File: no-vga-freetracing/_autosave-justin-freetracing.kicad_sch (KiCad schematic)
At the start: 121 parts, among them J1 DB15_Female_HighDensity, J2 Conn_02x03_Odd_Even, J3 Conn_01x08_MountingPin, J5 Barrel_Jack_Switch_Pin3Ring, K1 SW_Push, K10 SW_Push, K11 SW_Push, K12 SW_Push, K13 SW_Push, K14 SW_Push, K15 SW_Push, K16 SW_Push, K17 SW_Push, K18 SW_Push, K19 SW_Push, K2 SW_Push, K20 SW_Push, K21 SW_Push, K22 SW_Push, K23 SW_Push, K24 SW_Push, K25 SW_Push, K26 SW_Push, K27 SW_Push, K28 SW_Push, K29 SW_Push, K3 SW_Push, K30 SW_Push, K31 SW_Push, K32 SW_Push, K33 SW_Push, K34 SW_Push, K35 SW_Push, K36 SW_Push, K37 SW_Push, K38 SW_Push, K39 SW_Push, K4 SW_Push, K40 SW_Push, K41 SW_Push, K42 SW_Push, K43 SW_Push, K44 SW_Push, K45 SW_Push, K46 SW_Push, K47 SW_Push, K48 SW_Push, K49 SW_Push, K5 SW_Push, K6 SW_Push, K7 SW_Push, K8 SW_Push, K9 SW_Push, U1 ATmega1284-P, U2 ICE40UL1K-SWG16, Y1 20MHz

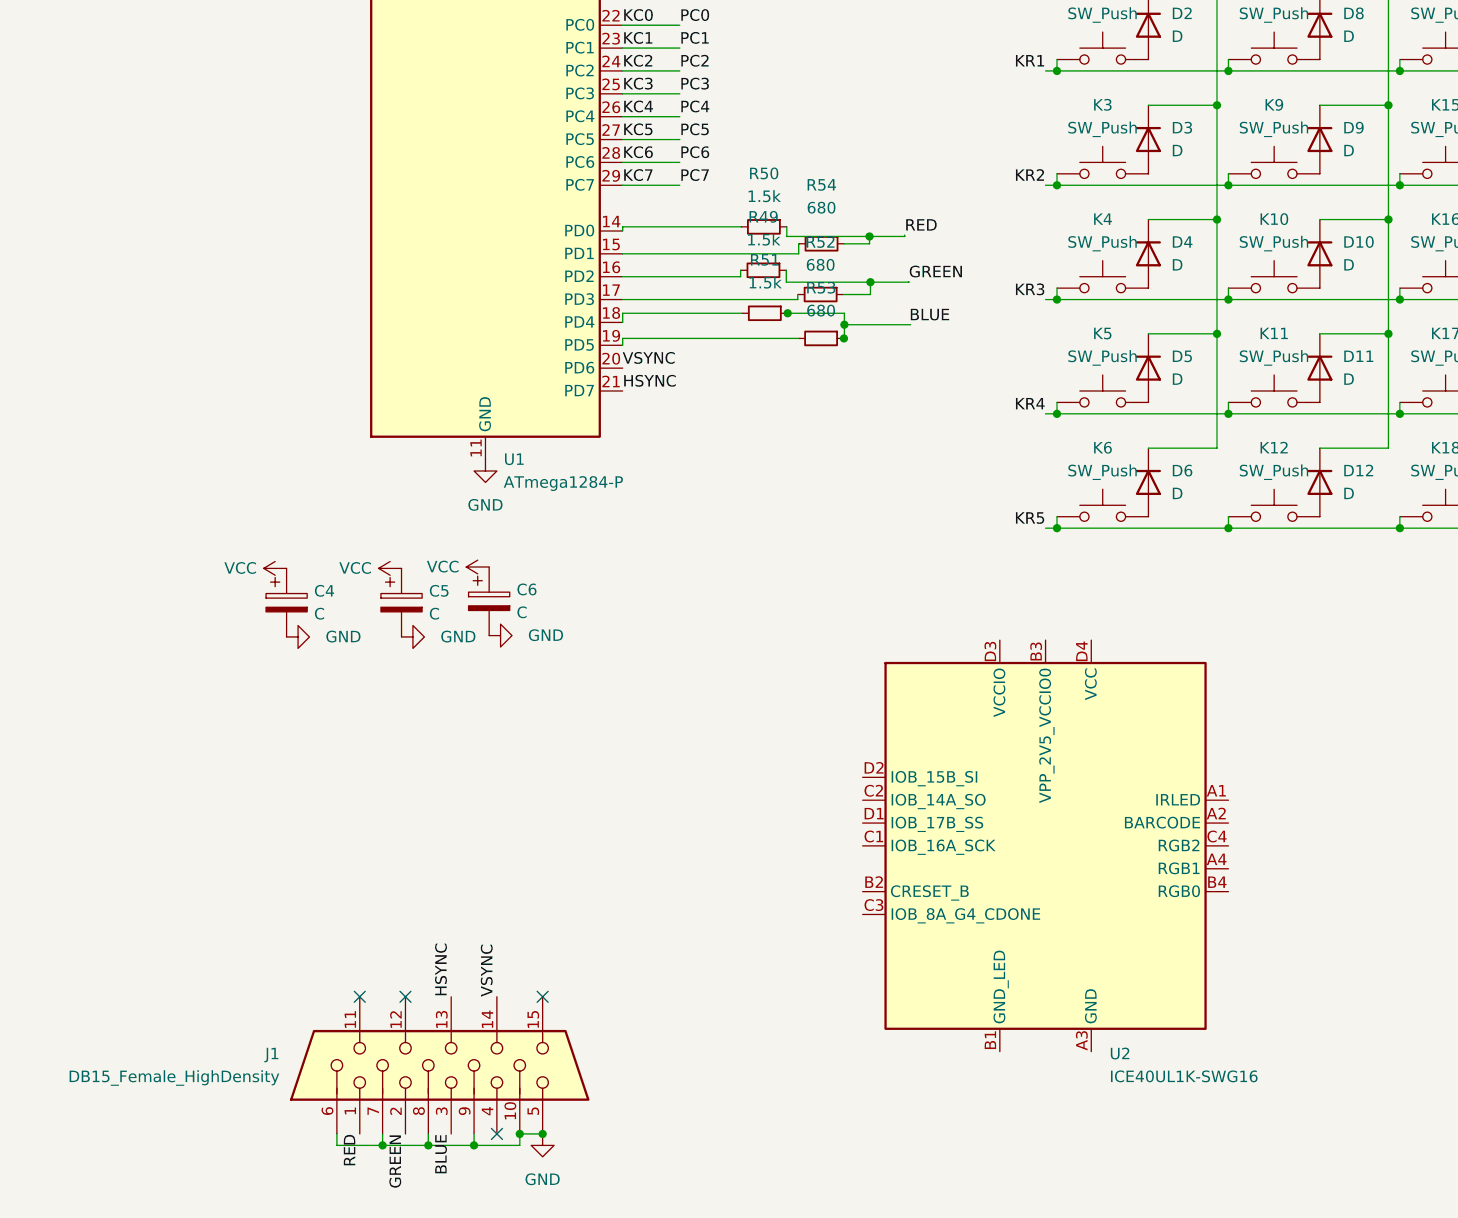
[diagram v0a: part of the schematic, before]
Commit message: Additional
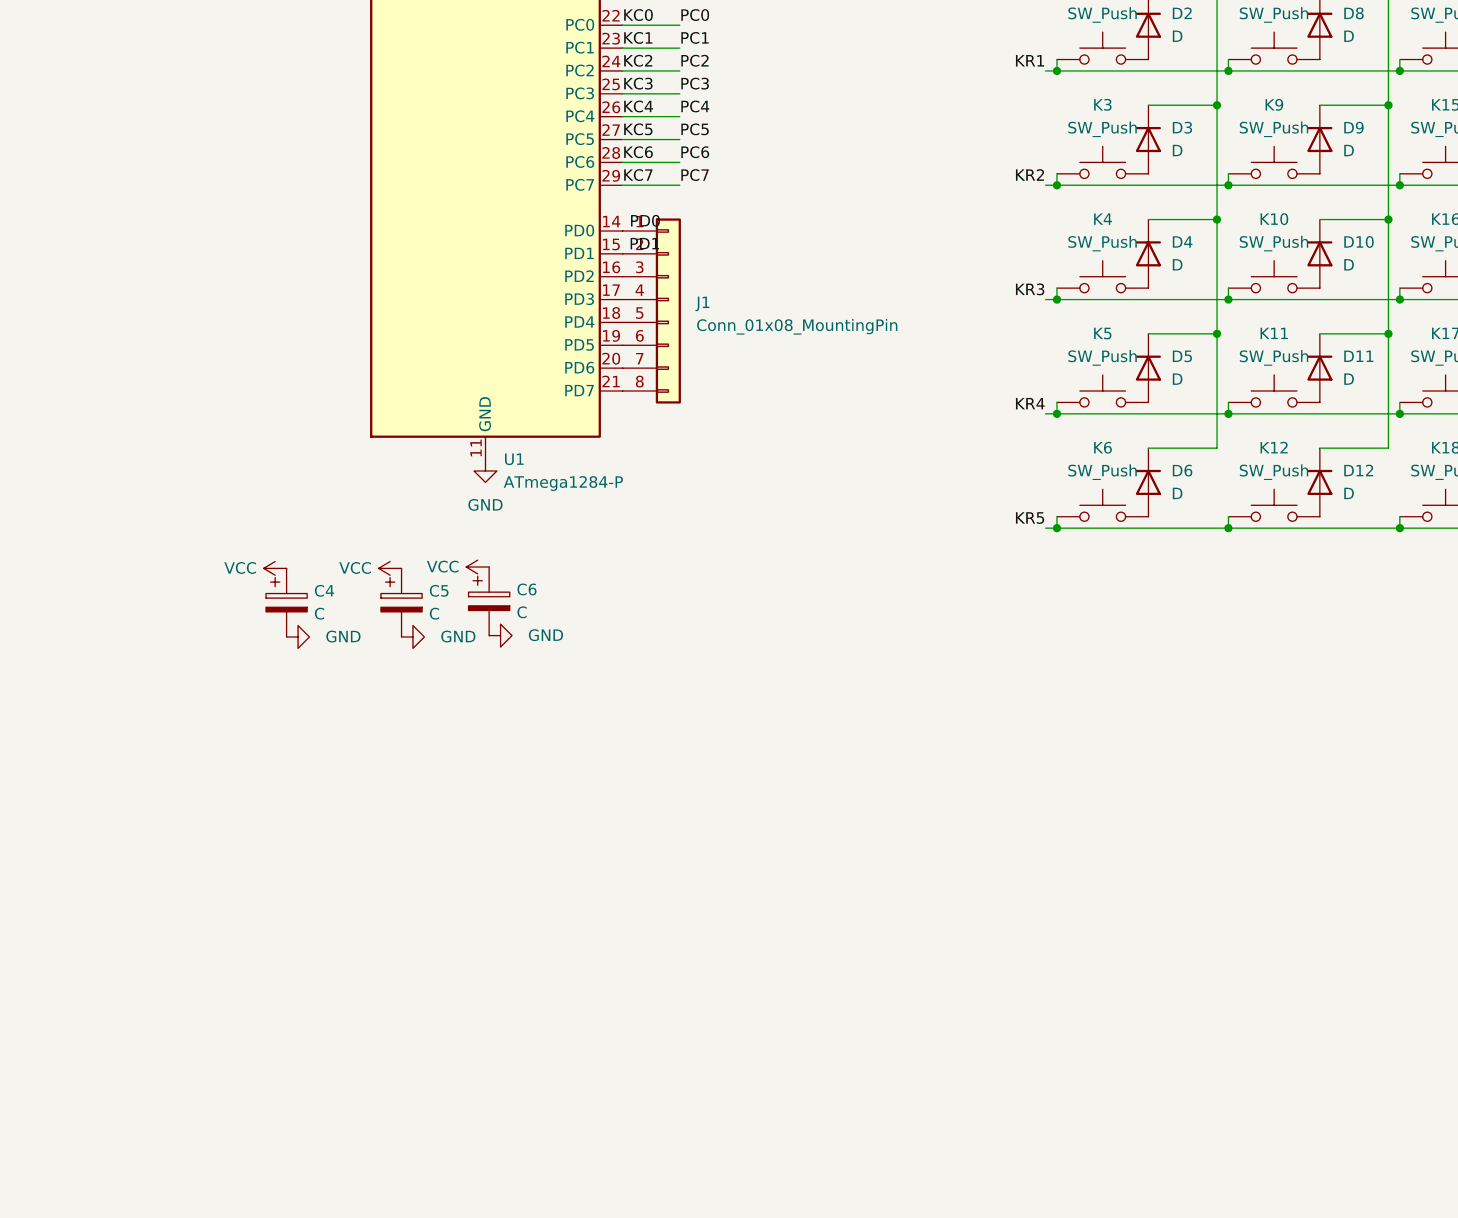
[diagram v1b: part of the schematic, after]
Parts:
- removed J1: DB15_Female_HighDensity, Connector_Dsub:DSUB-15_Female_Horizontal_P2.77x2.54mm_EdgePinOffset9.40mm, symbol Connector:DB15_Female_HighDensity
- removed R49, R50, R51: 1.5k, Resistor_THT:R_Axial_DIN0204_L3.6mm_D1.6mm_P5.08mm_Horizontal, symbol Device:R_Small
- removed R52, R53, R54: 680, Resistor_THT:R_Axial_DIN0204_L3.6mm_D1.6mm_P5.08mm_Horizontal, symbol Device:R_Small
- removed U2: ICE40UL1K-SWG16, Package_CSP:WLCSP-16_1.409x1.409mm_P0.35mm, symbol FPGA_Lattice:ICE40UL1K-SWG16
- added J1: Conn_01x08_MountingPin, Connector_PinHeader_2.54mm:PinHeader_1x08_P2.54mm_Vertical, symbol Connector_Generic:Conn_01x08
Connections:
- net at U1.19 (PD5): now also J1.6 (Pin_6)
- net at U1.17 (PD3): now also J1.4 (Pin_4)
- net at U1.14 (PD0): now also J1.1 (Pin_1)
- net at U1.15 (PD1): now also J1.2 (Pin_2)
- net at U1.16 (PD2): now also J1.3 (Pin_3)
- net at U1.18 (PD4): now also J1.5 (Pin_5)
- net HSYNC: no longer names the net of U1.21 (PD7)
- net HSYNC: now also J1.8 (Pin_8)
- net VSYNC: no longer names the net of U1.20 (PD6)
- net VSYNC: now also J1.7 (Pin_7)
- no-connect marks 5 -> 1
